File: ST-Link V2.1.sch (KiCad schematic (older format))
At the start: 50 parts, among them J1 Conn_01x08, J2 USB_OTG, J3 Conn_01x05, J4 Conn_01x08, Q1 MMBT3904, U0 stm32, U1 MIC5219-3.3, X1 8MHz

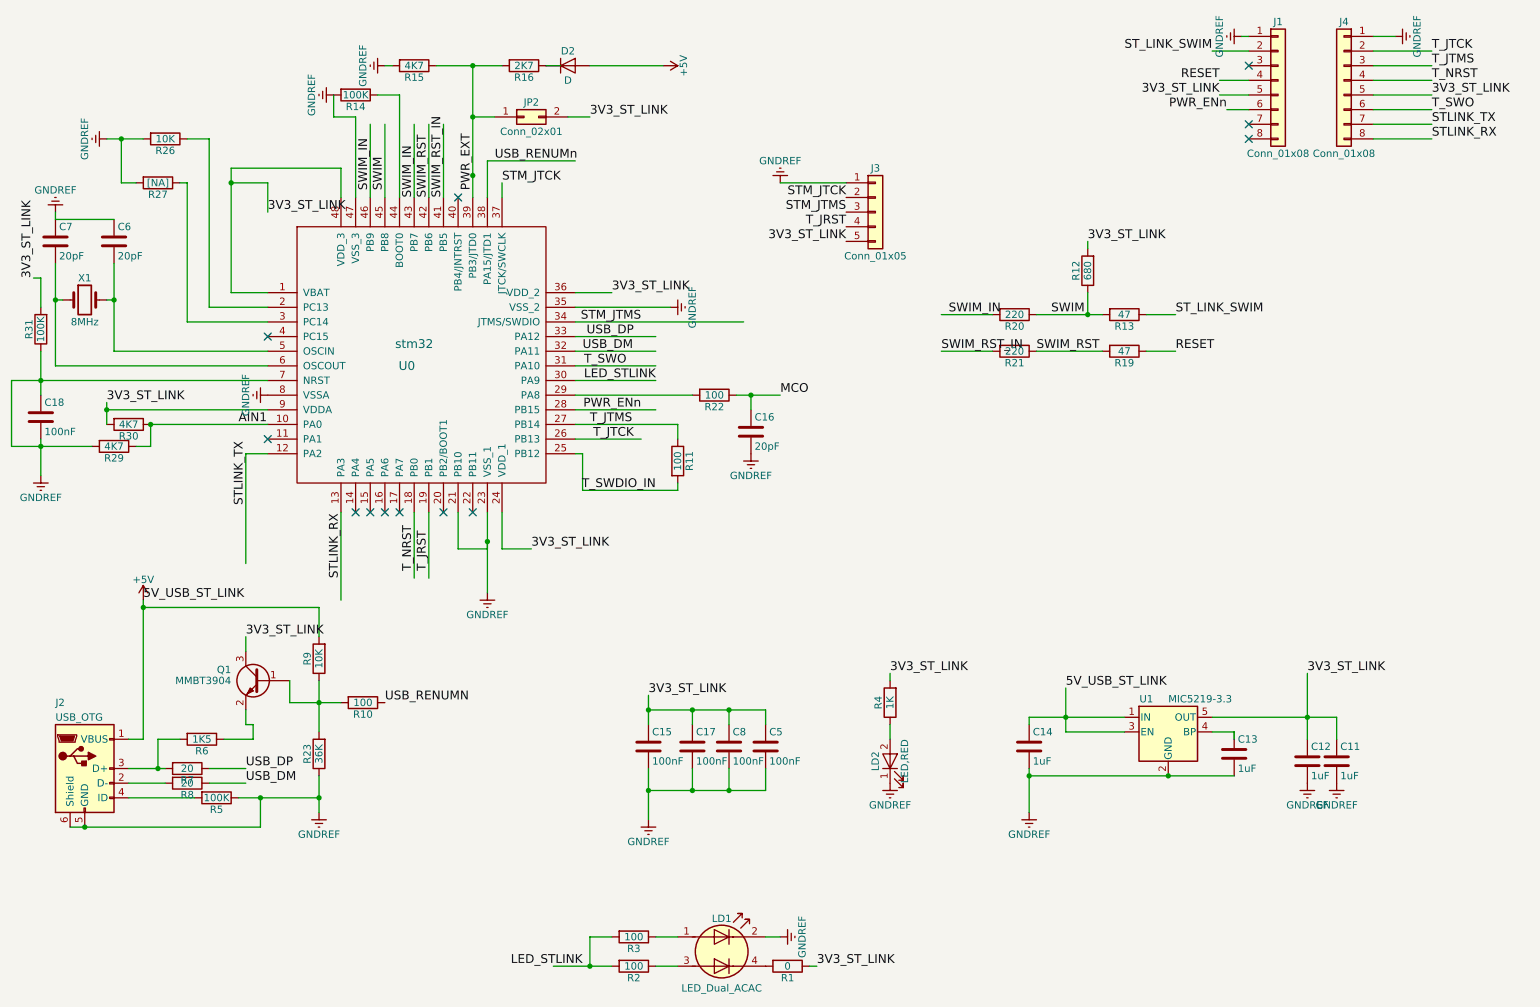
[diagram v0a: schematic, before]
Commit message: ALLIGNING
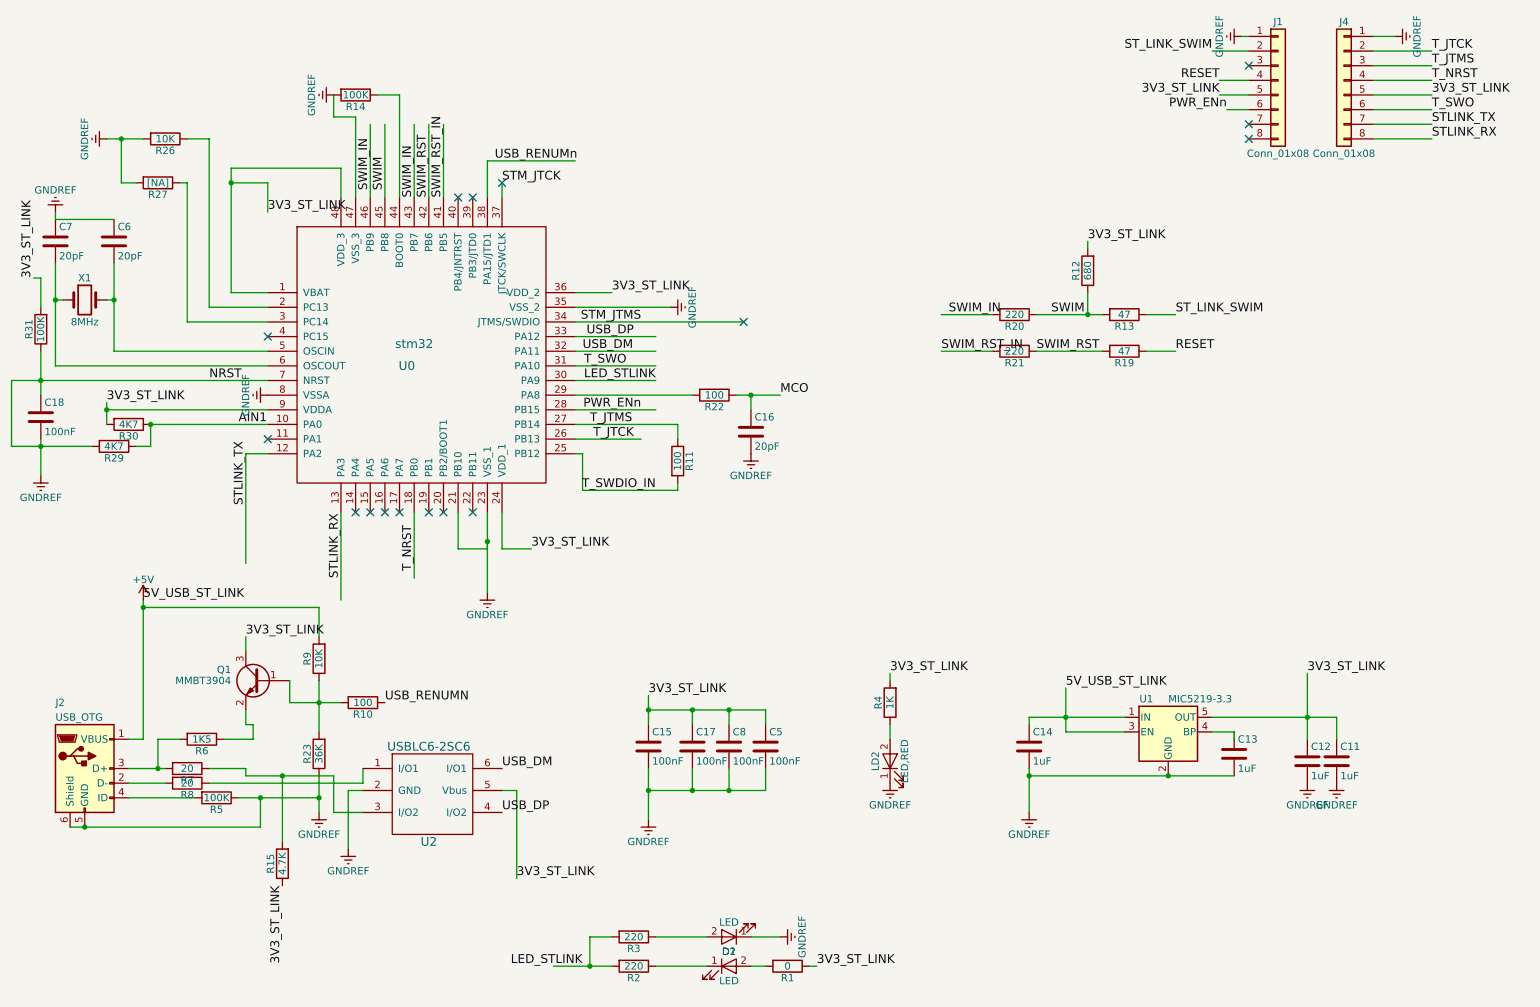
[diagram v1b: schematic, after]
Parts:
- removed D2: D, symbol D
- removed J3: Conn_01x05, symbol Conn_01x05
- removed JP2: Conn_02x01, symbol Conn_02x01
- removed LD1: LED_Dual_ACAC, symbol LED_Dual_ACAC
- removed R16: 2K7, symbol R
- added D1, D2: LED, LEDs:LED_0603, symbol LED
- added U2: USBLC6-2SC6, symbol USBLC6-2SC6
- C11, C12, C13, C14, C15, C16, C17, C18, C5, C6, C7, C8: footprint (none) -> Capacitors_SMD:C_0603
- J1, J4: footprint (none) -> Socket_Strips:Socket_Strip_Angled_1x08_Pitch2.54mm
- J2: footprint (none) -> Connectors_USB:USB_Micro-B_Molex-105017-0001
- LD2: footprint (none) -> LEDs:LED_0603
- R1, R10, R11, R12, R13, R14, R19, R20, R21, R22, R23, R26, R27, R29, R30, R31, R4, R5, R6, R7, R8, R9: footprint (none) -> Resistors_SMD:R_0603_HandSoldering
- R15: value 4K7 -> 4.7K; footprint (none) -> Resistors_SMD:R_0603_HandSoldering
- R2, R3: value 100 -> 220; footprint (none) -> Resistors_SMD:R_0603_HandSoldering
- U0: footprint (none) -> UFQFPN48:UFQFPN48
- X1: footprint (none) -> Crystals:Crystal_HC49-4H_Vertical
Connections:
- net labels added: NRST
- net labels removed: PWR_EXT, T_JRST
- wire segments 159 -> 161
- no-connect marks 12 -> 16
